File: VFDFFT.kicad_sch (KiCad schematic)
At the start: 261 parts, among them J1 USB_C_Receptacle_USB2.0, J10 Conn_01x02_Pin, J11 Conn_01x02_Male, J12 Conn_01x02_Male, J13 Conn_01x02_Male, J2 BATT, J3 FILAMENT+, J4 VFD_SIG, J5 USB_A, J6 Conn_01x03_Socket, J7 Conn_01x03_Socket, J8 Conn_01x02_Pin, J9 Conn_01x02_Pin, Q1 IRL7486MTRPBF, Q10 AO3400A, Q11 AO3400A, Q12 FS5N10S, Q2 ASDM30DN40E, Q3 ASDM30DN40E, Q4 HSCB2903, Q5 HSCB2903, Q6 AP6800, Q7 FS5N10S, Q8 FS5N10S, Q9 AO3400A, U1 IP2368, U10 TPS61170, U11 TPS61170, U12 W25Q128JVS, U13 TPS62170DSG, U14 LM358, U15 LM324, U16 LM3478, U17 LM2738, U18 LTC1446, U2 78L05_SOT23, U3 TPS40305, U4 LM3478, U5 LM3478, U6 STM32F446VETx, U7 AP6181, U8 HDC1080, U9 OPT3001DNPR, X1 SX1M32.768KM10F30TNN, Y1 26M, Y2 24M

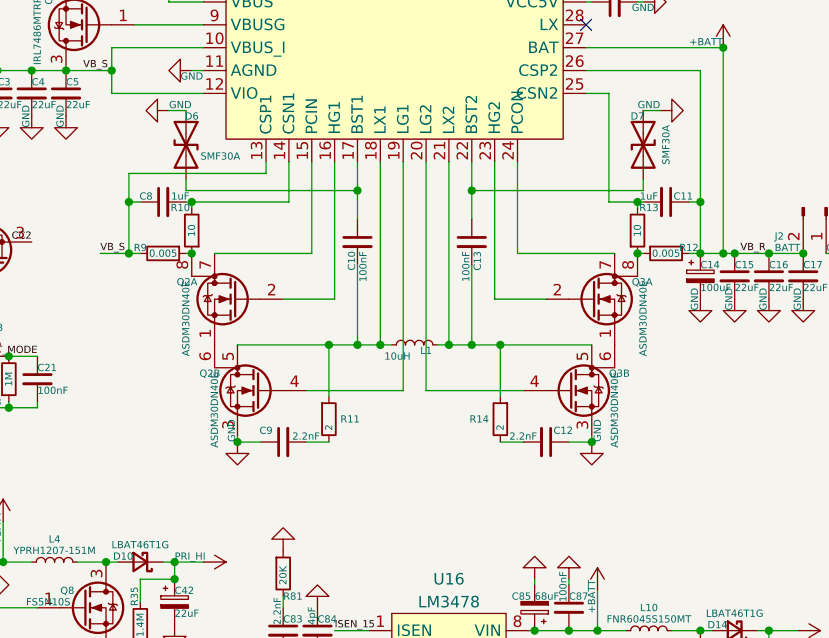
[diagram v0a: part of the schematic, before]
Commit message: file sync
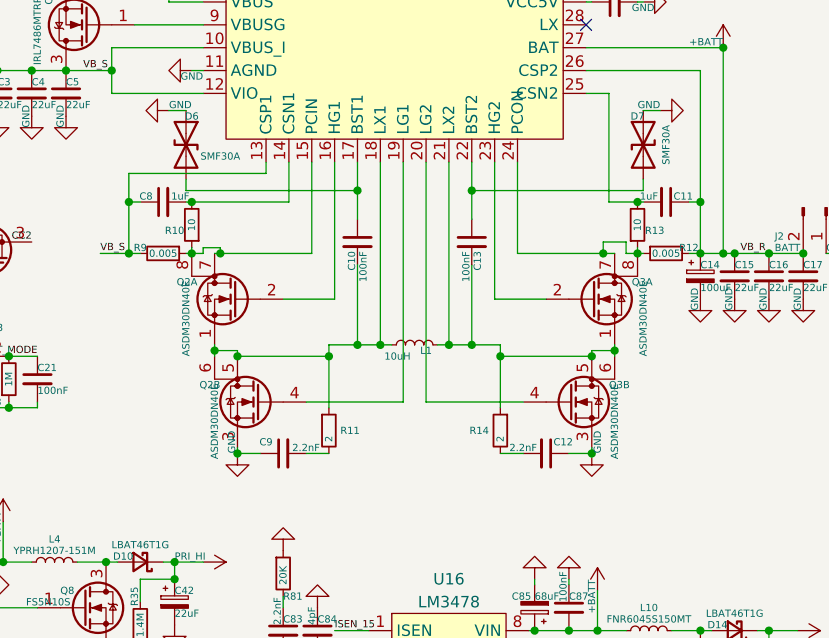
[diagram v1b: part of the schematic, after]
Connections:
- net at C10.2, L1.1, Q2.5 (D)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: now also Q2.1 (S), Q2.6 (D)
- net at Q2.7 (D), U1.15 (PCIN): now also Q2.8 (D), R10.1, R9.1
- net at C13.2, L1.2, Q3.5 (D)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: now also Q3.1 (S), Q3.6 (D)
- net at Q3.8 (D), R12.1, R13.1: now also Q3.7 (D), U1.24 (PCON)
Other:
- moved on the sheet: C12, C9, Q2B, Q3B, R10, R11, R13, R14
